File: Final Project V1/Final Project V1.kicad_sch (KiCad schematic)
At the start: 4 parts, among them U1 AP2112K-3.3, U2 ESP32-S3-WROOM-1

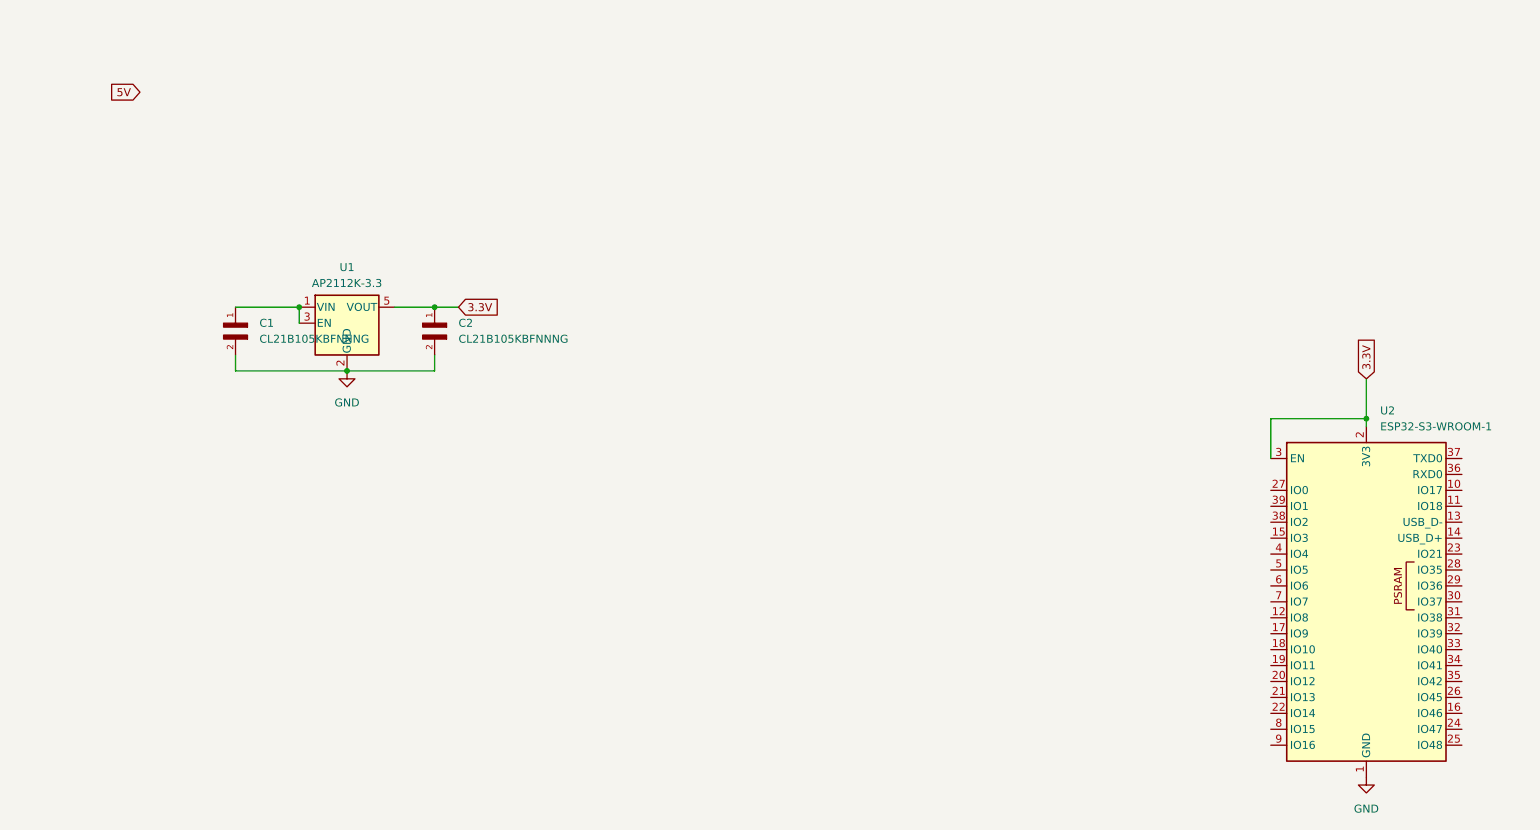
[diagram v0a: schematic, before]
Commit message: Finish power rail
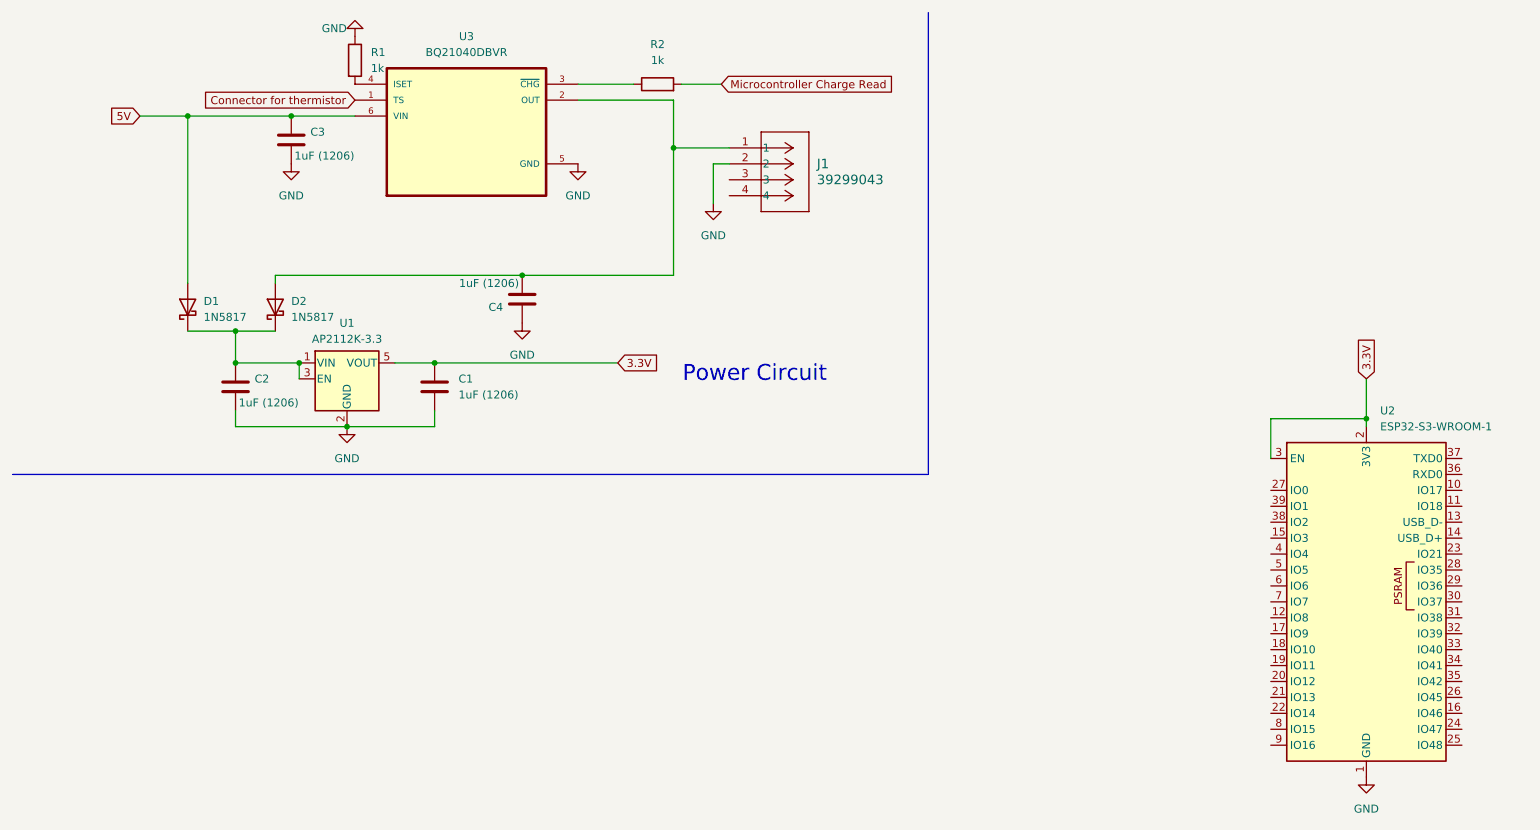
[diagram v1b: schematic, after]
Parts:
- removed C1, C2: CL21B105KBFNNNG, CL21B105KBFNNNG:CAPC2012X140N, symbol CL21B105KBFNNNG:CL21B105KBFNNNG
- added C1, C2, C3, C4: 1uF (1206), Capacitor_SMD:C_1206_3216Metric_Pad1.33x1.80mm_HandSolder, symbol Device:C
- added D1, D2: 1N5817, Diode_THT:D_DO-41_SOD81_P10.16mm_Horizontal, symbol Diode:1N5817
- added J1: 39299043, CONN_5566-04x2_MOL, symbol 39299043:39299043
- added R1, R2: 1k, Resistor_SMD:R_1206_3216Metric_Pad1.30x1.75mm_HandSolder, symbol Device:R
- added U3: BQ21040DBVR, BQ21040DBVR:SOT95P280X145-6N, symbol BQ21040DBVR:BQ21040DBVR
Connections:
- net 3.3V: now also C1.1
- net 5V: now also C3.1, D1.2 (A), U3.6 (VIN)
- net GND: now also C1.2, C2.2, C3.2, C4.1, J1.2, R1.1, U3.5 (GND)
- net at U1.1 (VIN), U1.3 (EN): now also C2.1, D1.1 (K), D2.1 (K)
- new net: C4.2, D2.2 (A), J1.1, U3.2 (OUT)
- new net: R1.2, U3.4 (ISET)
- new net: R2.1, U3.3 (~{CHG})
- new net Connector for thermistor: U3.1 (TS)
- new net Microcontroller Charge Read: R2.2
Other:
- note added: "Power Circuit"
- moved on the sheet: U1
